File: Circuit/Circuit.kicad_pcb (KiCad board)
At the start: 2 copper layers, 64.1 x 49.6 mm, 22 parts, among them SW1 SW_DPDT_x2, SW3 SW_DPDT_x2, U1 L7805

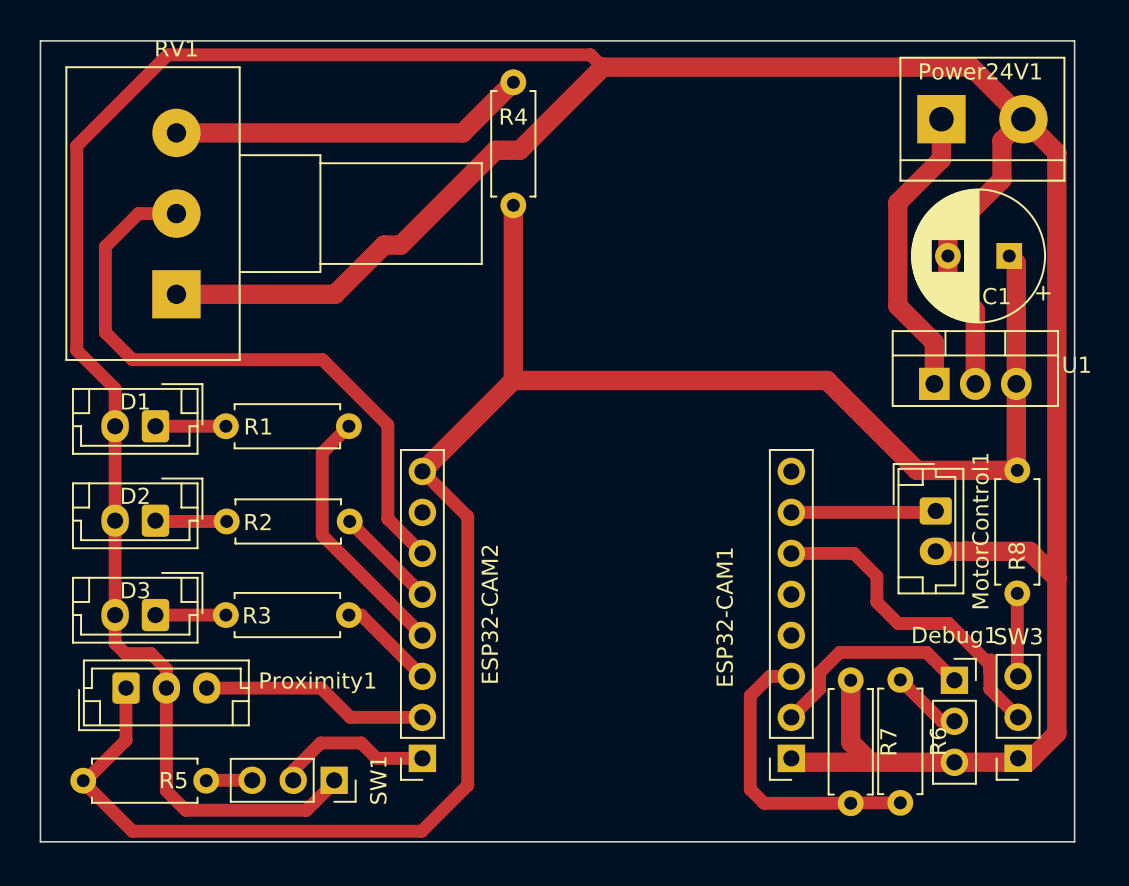
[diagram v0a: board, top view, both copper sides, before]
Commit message: schematic and PCB modification Done
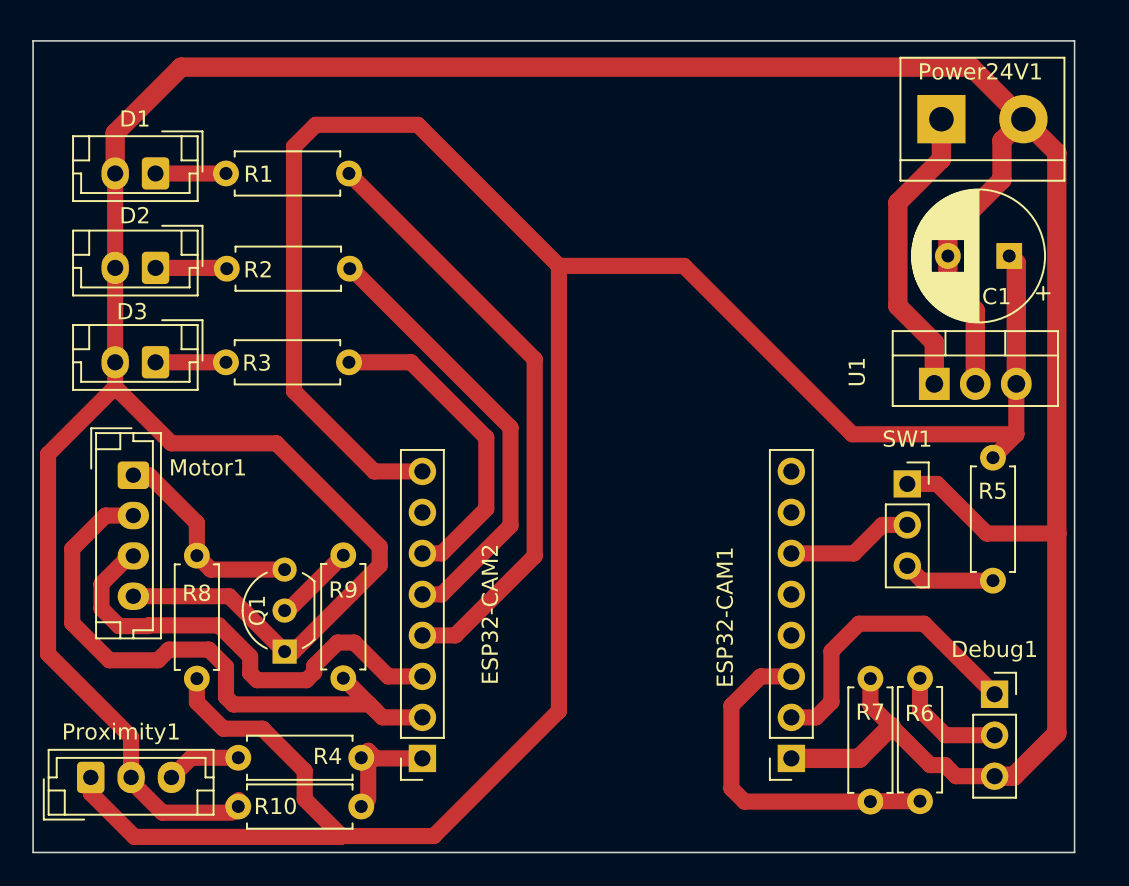
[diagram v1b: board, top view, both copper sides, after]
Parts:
- removed MotorControl1: JST-2P, Connector_JST:JST_EH_B2B-EH-A_1x02_P2.50mm_Vertical
- removed RV1: R_Potentiometer, Potentiometer_THT:Potentiometer_Alps_RK163_Single_Horizontal
- removed SW3: SW_DPDT_x2, Connector_PinSocket_2.54mm:PinSocket_1x03_P2.54mm_Vertical
- added Motor1: JST 4P, Connector_JST:JST_EH_B4B-EH-A_1x04_P2.50mm_Vertical, F.Cu at (128.8, 85.1)
- added Q1: S8050, Package_TO_SOT_THT:TO-92_Inline_Wide, F.Cu at (138.2, 96.0)
- added R10: 2k, Resistor_THT:R_Axial_DIN0207_L6.3mm_D2.5mm_P7.62mm_Horizontal, F.Cu at (135.3, 105.6)
- added R9: 1k, Resistor_THT:R_Axial_DIN0207_L6.3mm_D2.5mm_P7.62mm_Horizontal, F.Cu at (141.8, 97.7)
- Proximity1: value JST-3p -> JST 3P
- R4: value ?? -> 1k
- R6: value 330 -> 1k
- R7: value 330 -> 2k
- R8: value 10K -> 2k
- moved R8 50.9 mm to (132.8, 90.1), turned to -90 degrees
- moved R5 50.3 mm to (182.1, 91.6), turned to 90 degrees
- moved R4 42.9 mm to (143.0, 102.6), turned to 180 degrees
- moved SW1 40.0 mm to (176.8, 85.6), turned to 0 degrees
- moved D1 15.7 mm to (130.2, 66.4)
- moved D3 15.7 mm to (130.2, 78.1)
- moved R1 15.7 mm to (142.2, 66.4)
- moved R3 15.7 mm to (142.2, 78.1)
- moved D2 15.7 mm to (130.2, 72.3)
- moved R2 15.7 mm to (142.2, 72.3)
- moved Proximity1 5.95 mm to (126.2, 103.8)
- moved Debug1 2.63 mm to (182.2, 98.7)
- moved R6 1.22 mm to (177.6, 97.7)
- moved R7 1.22 mm to (174.5, 97.7)
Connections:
- ESP32-CAM1 pad 7: MotorPWM -> unconnected-(ESP32-CAM1-Pin_7-Pad7)
- ESP32-CAM2 pad 1: SWITCH1 -> Proximity
- ESP32-CAM2 pad 2: Proximity -> MotorDir1
- ESP32-CAM2 pad 3: GREEN_LED -> MotorPWM
- ESP32-CAM2 pad 6: POT_ADC -> GREEN_LED
- Proximity1 pad 3: Proximity -> Net-(Proximity1-Pin_3)
- R4 pad 1: Net-(R4-Pad1) -> Proximity
- R4 pad 2: +5V -> Net-(Proximity1-Pin_3)
- R8 pad 1: Net-(SW3A-C) -> MotorDir2
- SW1 pad 2: SWITCH1 -> BOOT_MODE
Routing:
- net +5V: track 119.6 -> 168.5 mm
- net POT_ADC: track 39.3 -> 0.00 mm
- net MotorDir1: track 0.00 -> 37.8 mm
- net Net-(R4-Pad1): track 22.2 -> 0.00 mm
- net RED_LED: track 16.2 -> 37.5 mm
- net YELLOW_LED: track 6.39 -> 27.3 mm
- net MotorPWM: track 8.99 -> 28.7 mm
- net GREEN_LED: track 6.13 -> 20.0 mm
- net MotorDir2: track 0.00 -> 13.0 mm
- net BOOT_MODE: track 20.8 -> 7.92 mm
- net SWITCH1: track 9.71 -> 0.00 mm
- net Proximity: track 14.1 -> 6.57 mm
- net TX: track 13.4 -> 18.7 mm
- net Net-(SW3A-C): track 5.16 -> 0.00 mm
- net Net-(Q1-B): track 0.00 -> 5.06 mm
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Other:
- board size 64.1 x 49.6 mm -> 64.5 x 50.3 mm
